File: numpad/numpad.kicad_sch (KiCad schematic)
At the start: 56 parts, among them SW1 SW_Push, U1 ATmega32U2-A, U2 PRTR5V0U2X, Y1 Crystal_GND24_Small

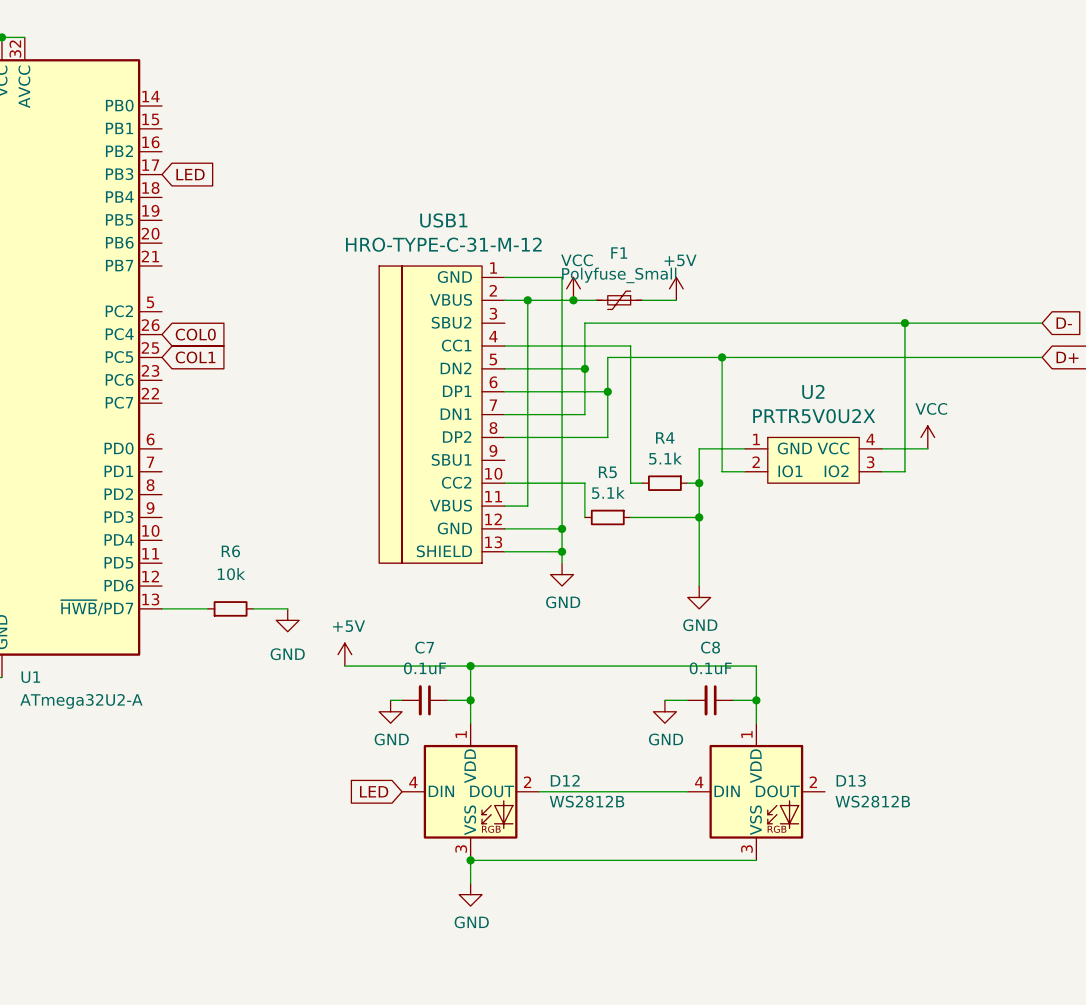
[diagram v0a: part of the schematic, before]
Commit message: finished keypad, needs cleaning up
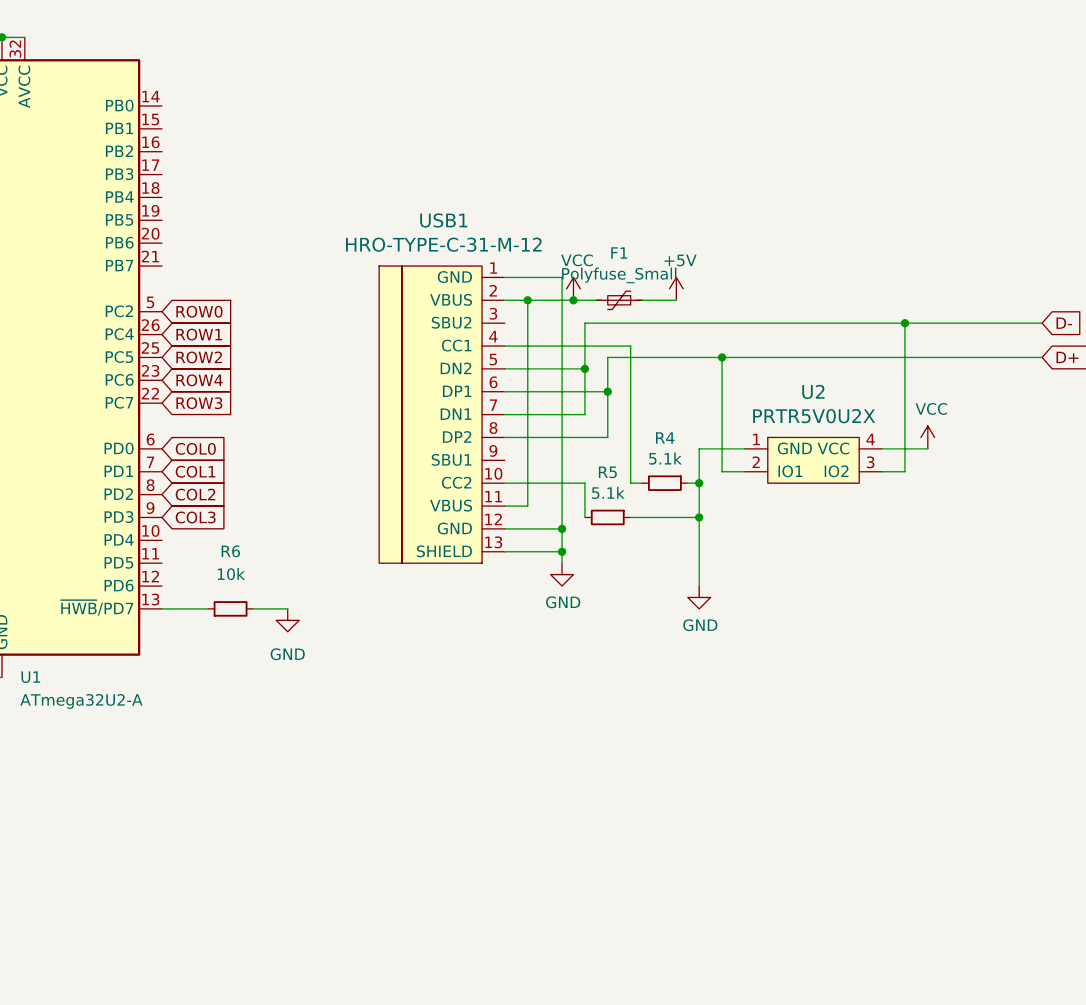
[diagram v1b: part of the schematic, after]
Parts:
- removed C7, C8: 0.1uF, Capacitor_SMD:C_0805_2012Metric_Pad1.18x1.45mm_HandSolder, symbol Device:C_Small
- removed D12, D13: WS2812B, LED_SMD:LED_WS2812B_PLCC4_5.0x5.0mm_P3.2mm, symbol LED:WS2812B
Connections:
- net COL0: now also U1.6 (PD0); no longer U1.26 (PC4)
- net COL1: now also U1.7 (PD1); no longer U1.25 (PC5)
- net COL2: now also U1.8 (PD2)
- net COL3: now also U1.9 (PD3)
- net ROW0: now also U1.5 (PC2)
- net ROW1: now also U1.26 (PC4)
- net ROW2: now also U1.25 (PC5)
- net ROW3: now also U1.22 (PC7)
- net ROW4: now also U1.23 (PC6)
- net LED: no longer names the net of U1.17 (PB3)

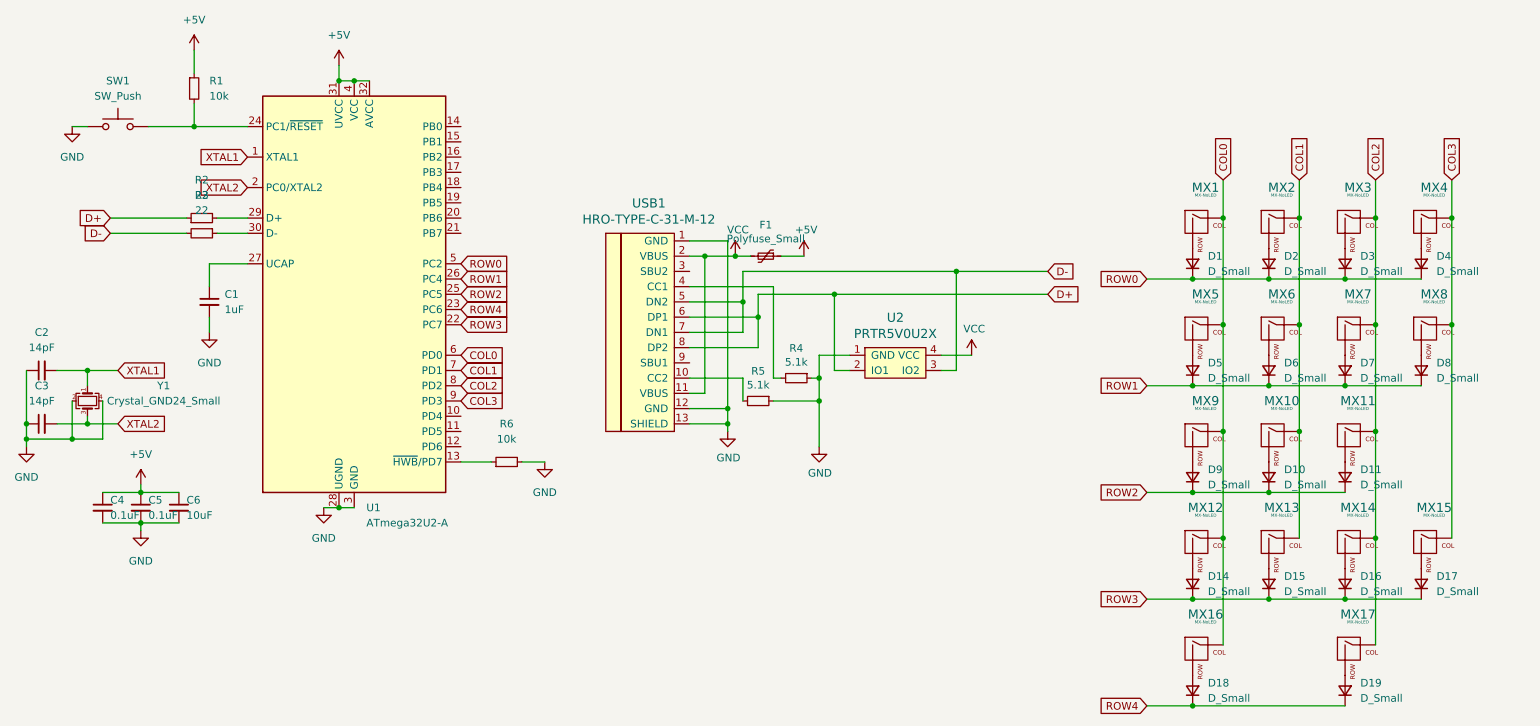
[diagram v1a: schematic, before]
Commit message: finished numpad pcb
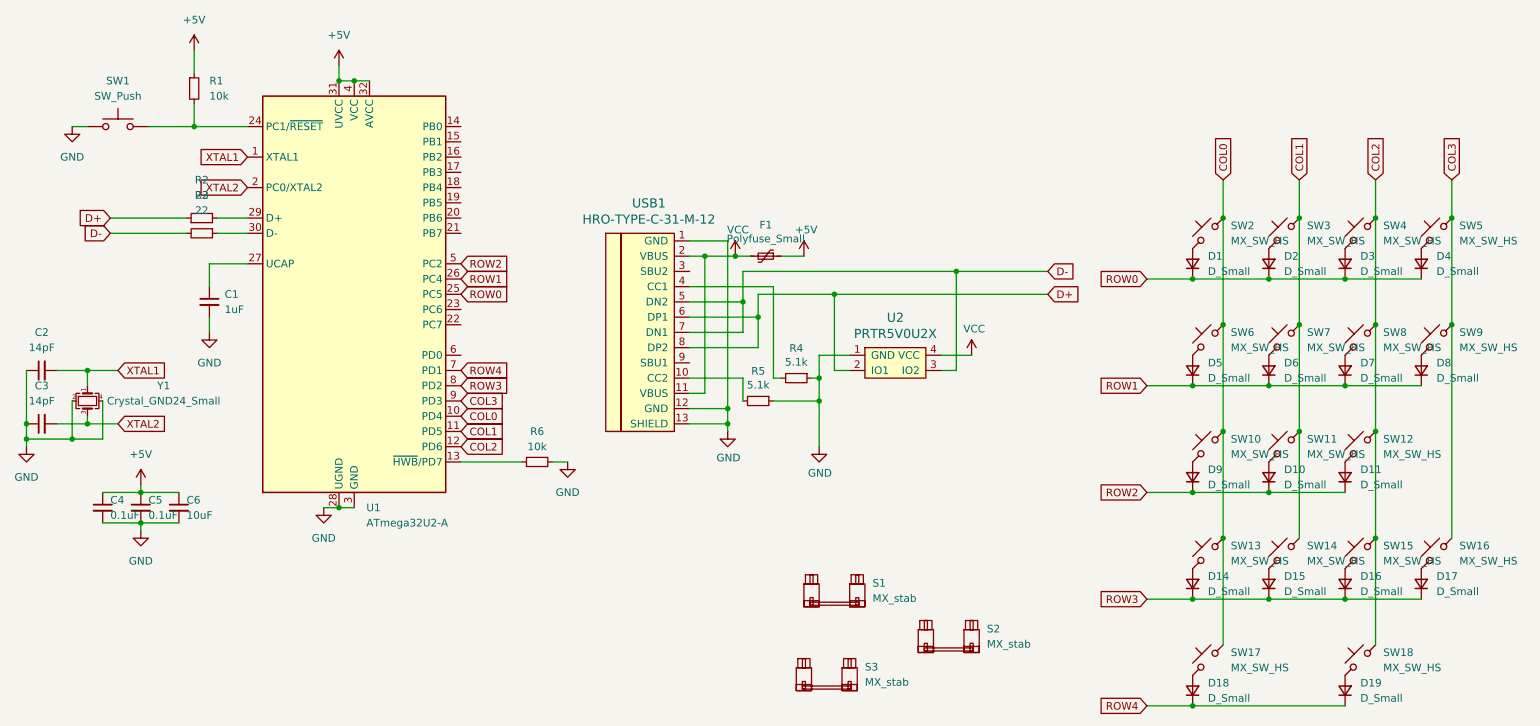
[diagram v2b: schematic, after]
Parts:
- removed MX1, MX10, MX11, MX12, MX13, MX14, MX17, MX2, MX3, MX4, MX5, MX6, MX7, MX9: MX-NoLED, MX_Only:MXOnly-1U-Hotswap, symbol MX_Alps_Hybrid:MX-NoLED
- removed MX15, MX16, MX8: MX-NoLED, MX_Only:MXOnly-2U-Hotswap, symbol MX_Alps_Hybrid:MX-NoLED
- added S1, S2, S3: MX_stab, marbastlib-mx:STAB_MX_2u, symbol marbastlib-mx:MX_stab
- added SW10, SW11, SW12, SW13, SW14, SW15, SW16, SW17, SW18, SW2, SW3, SW4, SW5, SW6, SW7, SW8, SW9: MX_SW_HS, marbastlib-mx:SW_MX_HS_1u, symbol marbastlib-mx:MX_SW_HS
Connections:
- net COL0: now also U1.10 (PD4), SW10.2, SW13.2, SW17.2, SW2.2, SW6.2; no longer U1.6 (PD0)
- net COL1: now also U1.11 (PD5), SW11.2, SW14.2, SW3.2, SW7.2; no longer U1.7 (PD1)
- net COL2: now also U1.12 (PD6), SW12.2, SW15.2, SW18.2, SW4.2, SW8.2; no longer U1.8 (PD2)
- net COL3: now also SW16.2, SW5.2, SW9.2
- net ROW0: now also U1.25 (PC5); no longer U1.5 (PC2)
- net ROW2: now also U1.5 (PC2); no longer U1.25 (PC5)
- net ROW3: now also U1.8 (PD2); no longer U1.22 (PC7)
- net ROW4: now also U1.7 (PD1); no longer U1.23 (PC6)
- net at D4.2 (A): now also SW5.1
- net at D10.2 (A): now also SW11.1
- net at D9.2 (A): now also SW10.1
- net at D5.2 (A): now also SW6.1
- net at D8.2 (A): now also SW9.1
- net at D16.2 (A): now also SW15.1
- net at D19.2 (A): now also SW18.1
- net at D18.2 (A): now also SW17.1
- net at D7.2 (A): now also SW8.1
- net at D2.2 (A): now also SW3.1
- net at D17.2 (A): now also SW16.1
- net at D3.2 (A): now also SW4.1
- net at D15.2 (A): now also SW14.1
- net at D11.2 (A): now also SW12.1
- net at D6.2 (A): now also SW7.1
- net at D14.2 (A): now also SW13.1
- net at D1.2 (A): now also SW2.1
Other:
- moved on the sheet: R6

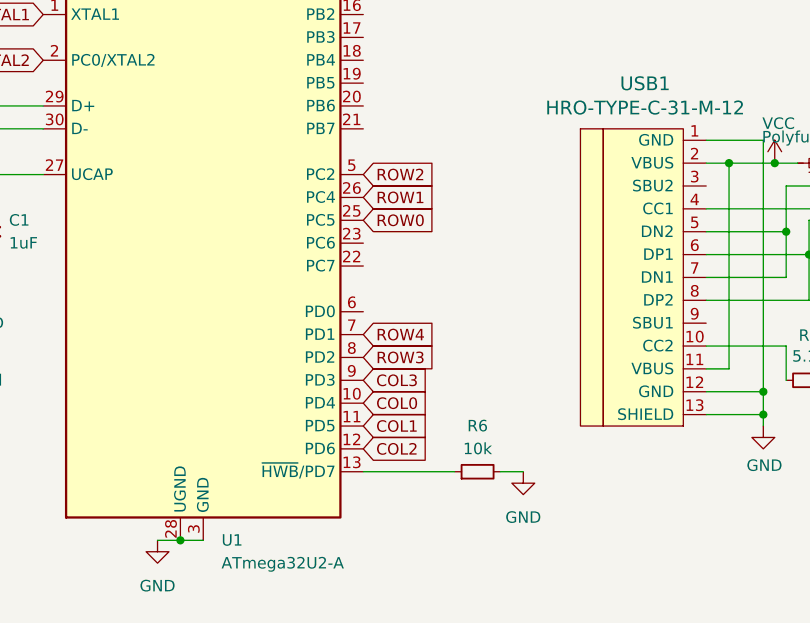
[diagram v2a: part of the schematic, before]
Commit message: did a bit of work 3d modelling today
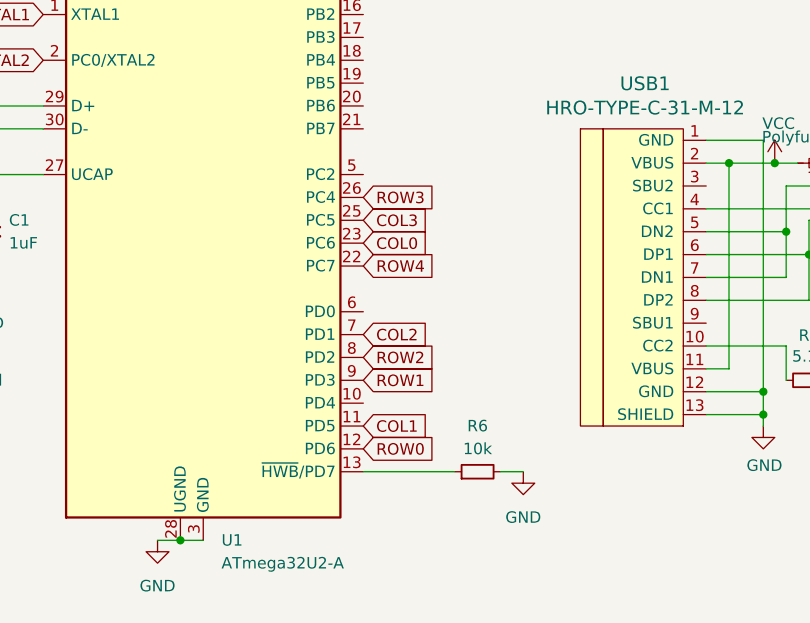
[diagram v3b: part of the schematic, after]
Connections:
- net COL0: now also U1.23 (PC6); no longer U1.10 (PD4)
- net COL2: now also U1.7 (PD1); no longer U1.12 (PD6)
- net COL3: now also U1.25 (PC5); no longer U1.9 (PD3)
- net ROW0: now also U1.12 (PD6); no longer U1.25 (PC5)
- net ROW1: now also U1.9 (PD3); no longer U1.26 (PC4)
- net ROW2: now also U1.8 (PD2); no longer U1.5 (PC2)
- net ROW3: now also U1.26 (PC4); no longer U1.8 (PD2)
- net ROW4: now also U1.22 (PC7); no longer U1.7 (PD1)
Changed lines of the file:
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@@
     )
   )
-  (global_label "ROW0" (shape input) (at 96.52 62.23 0) (fields_autoplaced)
+  (global_label "ROW0" (shape input) (at 96.52 87.63 0) (fields_autoplaced)
     (effects (font (size 1.27 1.27)) (justify left))
-    (property "Intersheet References" "${INTERSHEET_REFS}" (id 0) (at 104.1945 62.1506 0)
+    (property "Intersheet References" "${INTERSHEET_REFS}" (id 0) (at 104.1945 87.5506 0)
       (effects (font (size 1.27 1.27)) (justify left) hide)
     )
@@
     )
   )
-  (global_label "COL0" (shape input) (at 96.52 82.55 0) (fields_autoplaced)
+  (global_label "COL0" (shape input) (at 96.52 64.77 0) (fields_autoplaced)
     (effects (font (size 1.27 1.27)) (justify left))
-    (property "Intersheet References" "${INTERSHEET_REFS}" (id 0) (at 103.7712 82.4706 0)
+    (property "Intersheet References" "${INTERSHEET_REFS}" (id 0) (at 103.7712 64.6906 0)
       (effects (font (size 1.27 1.27)) (justify left) hide)
     )
   )
-  (global_label "COL3" (shape input) (at 96.52 80.01 0) (fields_autoplaced)
+  (global_label "COL3" (shape input) (at 96.52 62.23 0) (fields_autoplaced)
     (effects (font (size 1.27 1.27)) (justify left))
-    (property "Intersheet References" "${INTERSHEET_REFS}" (id 0) (at 103.7712 79.9306 0)
+    (property "Intersheet References" "${INTERSHEET_REFS}" (id 0) (at 103.7712 62.1506 0)
       (effects (font (size 1.27 1.27)) (justify left) hide)
     )
   )
-  (global_label "ROW1" (shape input) (at 96.52 59.69 0) (fields_autoplaced)
+  (global_label "ROW1" (shape input) (at 96.52 80.01 0) (fields_autoplaced)
     (effects (font (size 1.27 1.27)) (justify left))
-    (property "Intersheet References" "${INTERSHEET_REFS}" (id 0) (at 104.1945 59.6106 0)
+    (property "Intersheet References" "${INTERSHEET_REFS}" (id 0) (at 104.1945 79.9306 0)
       (effects (font (size 1.27 1.27)) (justify left) hide)
     )
@@
     )
   )
-  (global_label "ROW3" (shape input) (at 96.52 77.47 0) (fields_autoplaced)
+  (global_label "ROW3" (shape input) (at 96.52 59.69 0) (fields_autoplaced)
     (effects (font (size 1.27 1.27)) (justify left))
-    (property "Intersheet References" "${INTERSHEET_REFS}" (id 0) (at 104.1945 77.3906 0)
+    (property "Intersheet References" "${INTERSHEET_REFS}" (id 0) (at 104.1945 59.6106 0)
       (effects (font (size 1.27 1.27)) (justify left) hide)
     )
@@
     )
   )
-  (global_label "ROW2" (shape input) (at 96.52 57.15 0) (fields_autoplaced)
+  (global_label "ROW2" (shape input) (at 96.52 77.47 0) (fields_autoplaced)
     (effects (font (size 1.27 1.27)) (justify left))
-    (property "Intersheet References" "${INTERSHEET_REFS}" (id 0) (at 104.1945 57.0706 0)
+    (property "Intersheet References" "${INTERSHEET_REFS}" (id 0) (at 104.1945 77.3906 0)
       (effects (font (size 1.27 1.27)) (justify left) hide)
     )
@@
     )
   )
-  (global_label "ROW4" (shape input) (at 96.52 74.93 0) (fields_autoplaced)
+  (global_label "ROW4" (shape input) (at 96.52 67.31 0) (fields_autoplaced)
     (effects (font (size 1.27 1.27)) (justify left))
-    (property "Intersheet References" "${INTERSHEET_REFS}" (id 0) (at 104.1945 74.8506 0)
+    (property "Intersheet References" "${INTERSHEET_REFS}" (id 0) (at 104.1945 67.2306 0)
       (effects (font (size 1.27 1.27)) (justify left) hide)
     )
@@
     )
   )
-  (global_label "COL2" (shape input) (at 96.52 87.63 0) (fields_autoplaced)
+  (global_label "COL2" (shape input) (at 96.52 74.93 0) (fields_autoplaced)
     (effects (font (size 1.27 1.27)) (justify left))
-    (property "Intersheet References" "${INTERSHEET_REFS}" (id 0) (at 103.7712 87.5506 0)
+    (property "Intersheet References" "${INTERSHEET_REFS}" (id 0) (at 103.7712 74.8506 0)
       (effects (font (size 1.27 1.27)) (justify left) hide)
     )

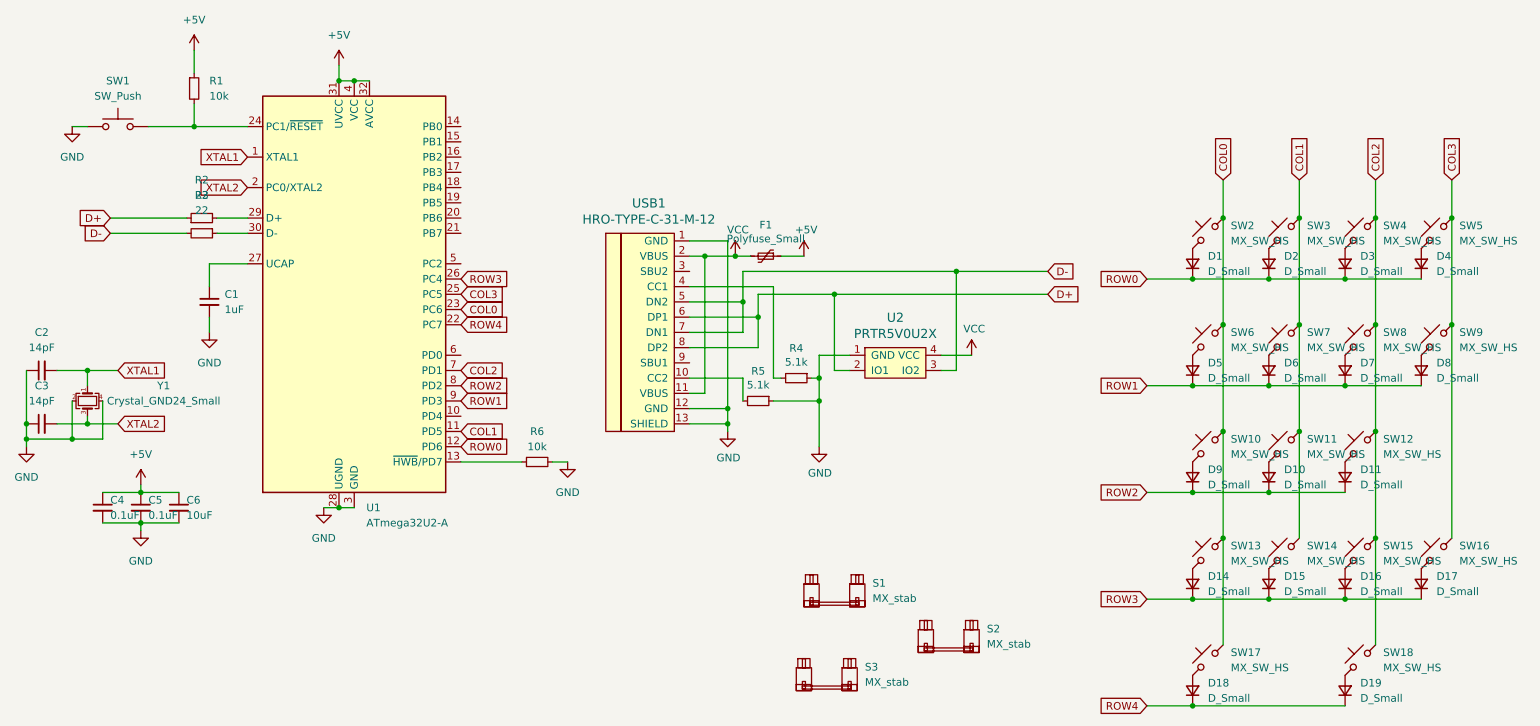
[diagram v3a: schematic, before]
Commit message: work
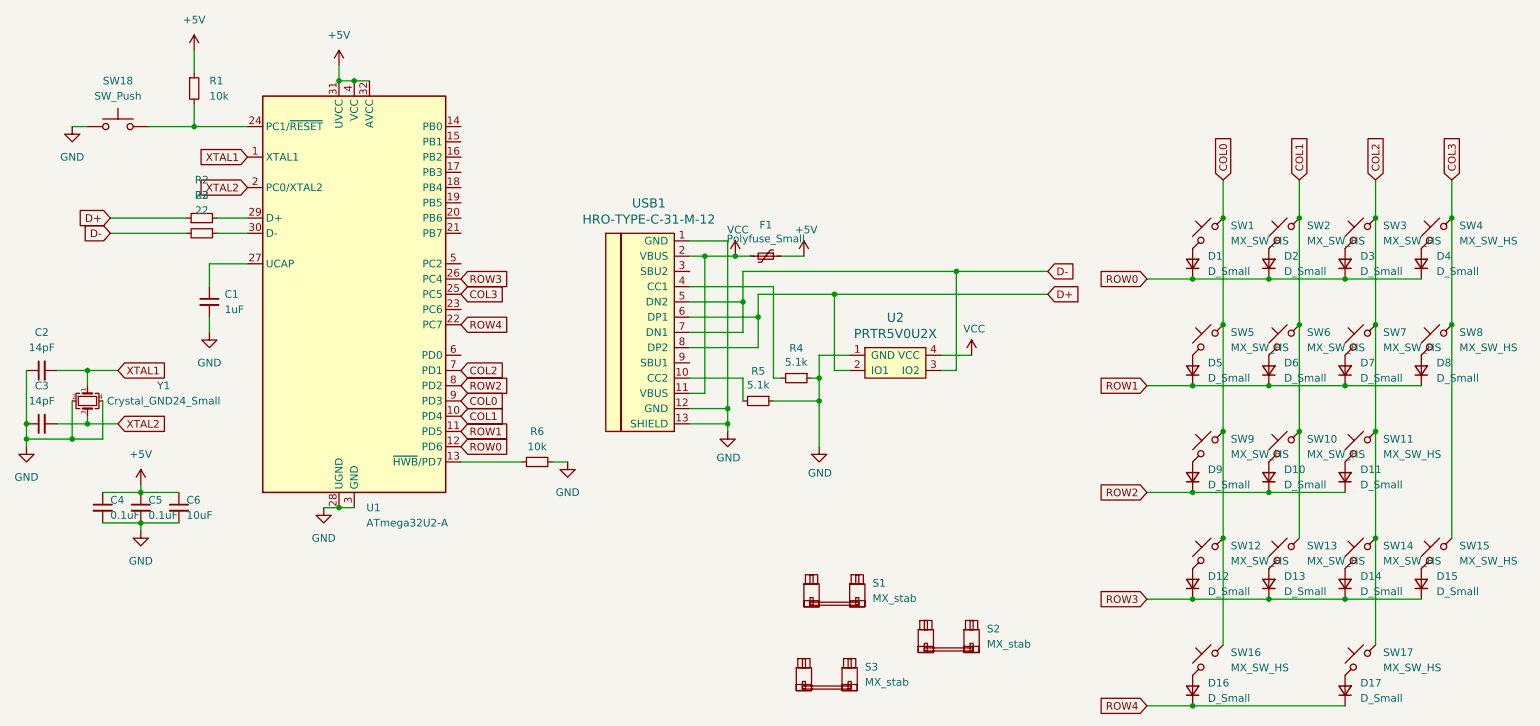
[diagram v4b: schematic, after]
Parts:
- renumbered D14 to D12, D15 to D13, D16 to D14, D17 to D15, D18 to D16, D19 to D17, SW2 to SW1, SW11 to SW10, SW12 to SW11, SW13 to SW12, SW14 to SW13, SW15 to SW14, SW16 to SW15, SW17 to SW16, SW18 to SW17, SW1 to SW18, SW3 to SW2, SW4 to SW3, SW5 to SW4, SW6 to SW5, SW7 to SW6, SW8 to SW7, SW9 to SW8, SW10 to SW9
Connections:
- net COL0: now also U1.9 (PD3); no longer U1.23 (PC6)
- net COL1: now also U1.10 (PD4); no longer U1.11 (PD5)
- net ROW1: now also U1.11 (PD5); no longer U1.9 (PD3)
